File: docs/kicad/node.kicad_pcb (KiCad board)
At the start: 2 copper layers, 181.1 x 116.5 mm, 8 parts, among them J10 Conn_01x04_Pin, J11 Conn_01x04_Pin, J9 Conn_01x08, U1 ESP32-DevKitC, U2 ESP32-DevKitC, U3 ESP32-DevKitC, U4 ESP32-DevKitC, U5 ESP32-DevKitC

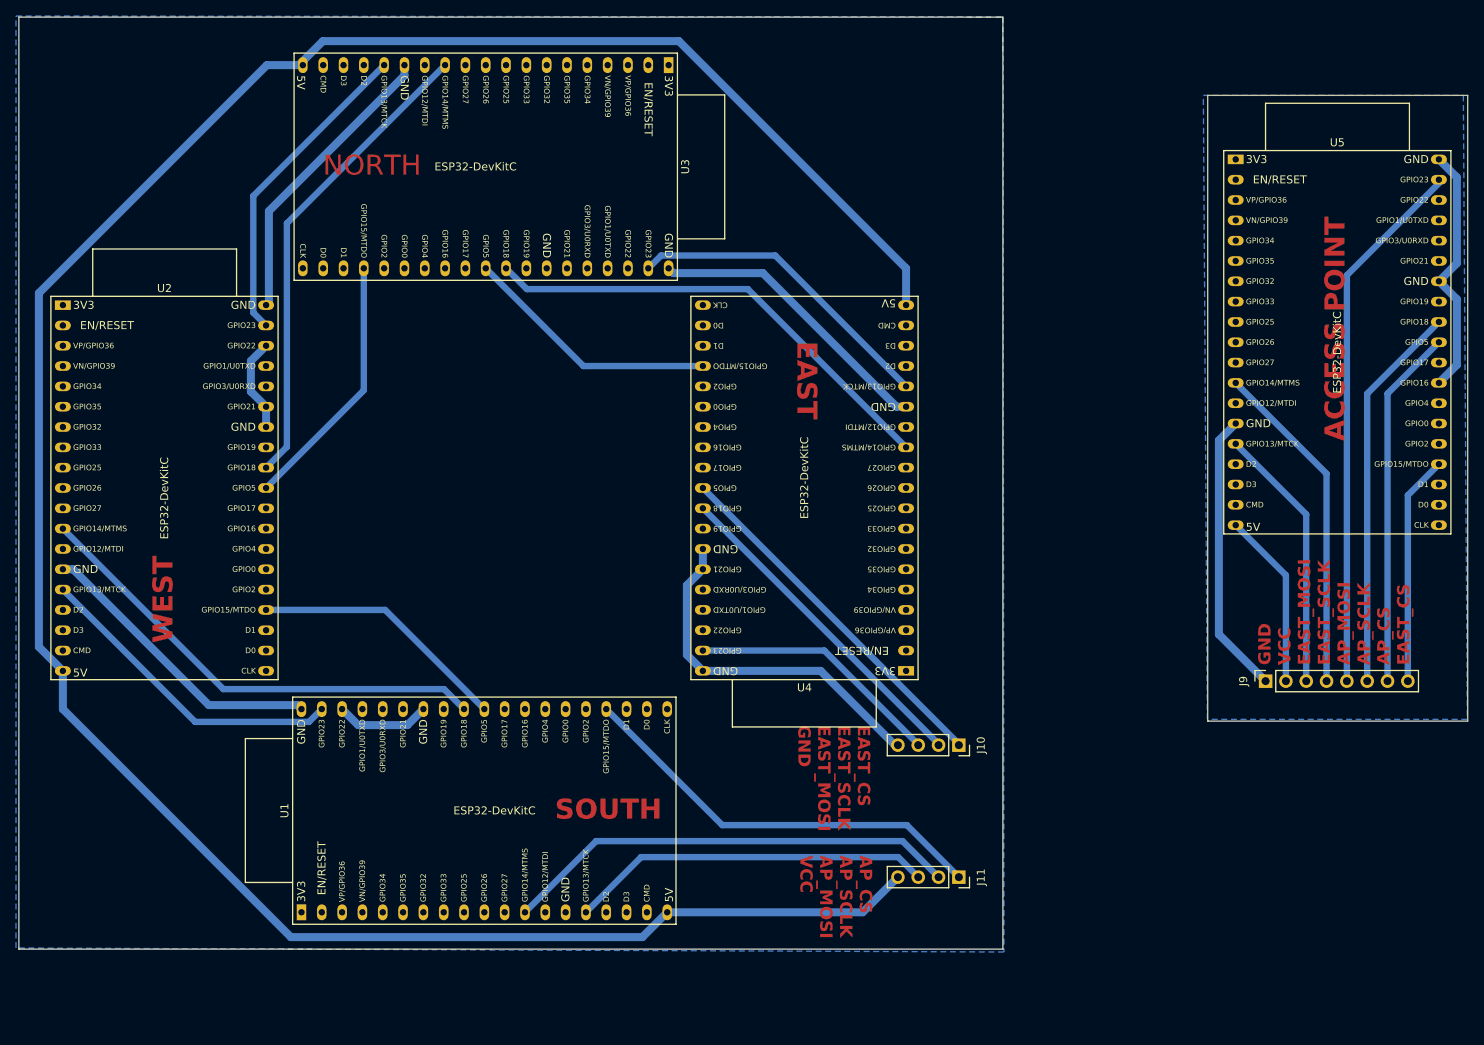
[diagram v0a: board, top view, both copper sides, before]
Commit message: resolved all errors
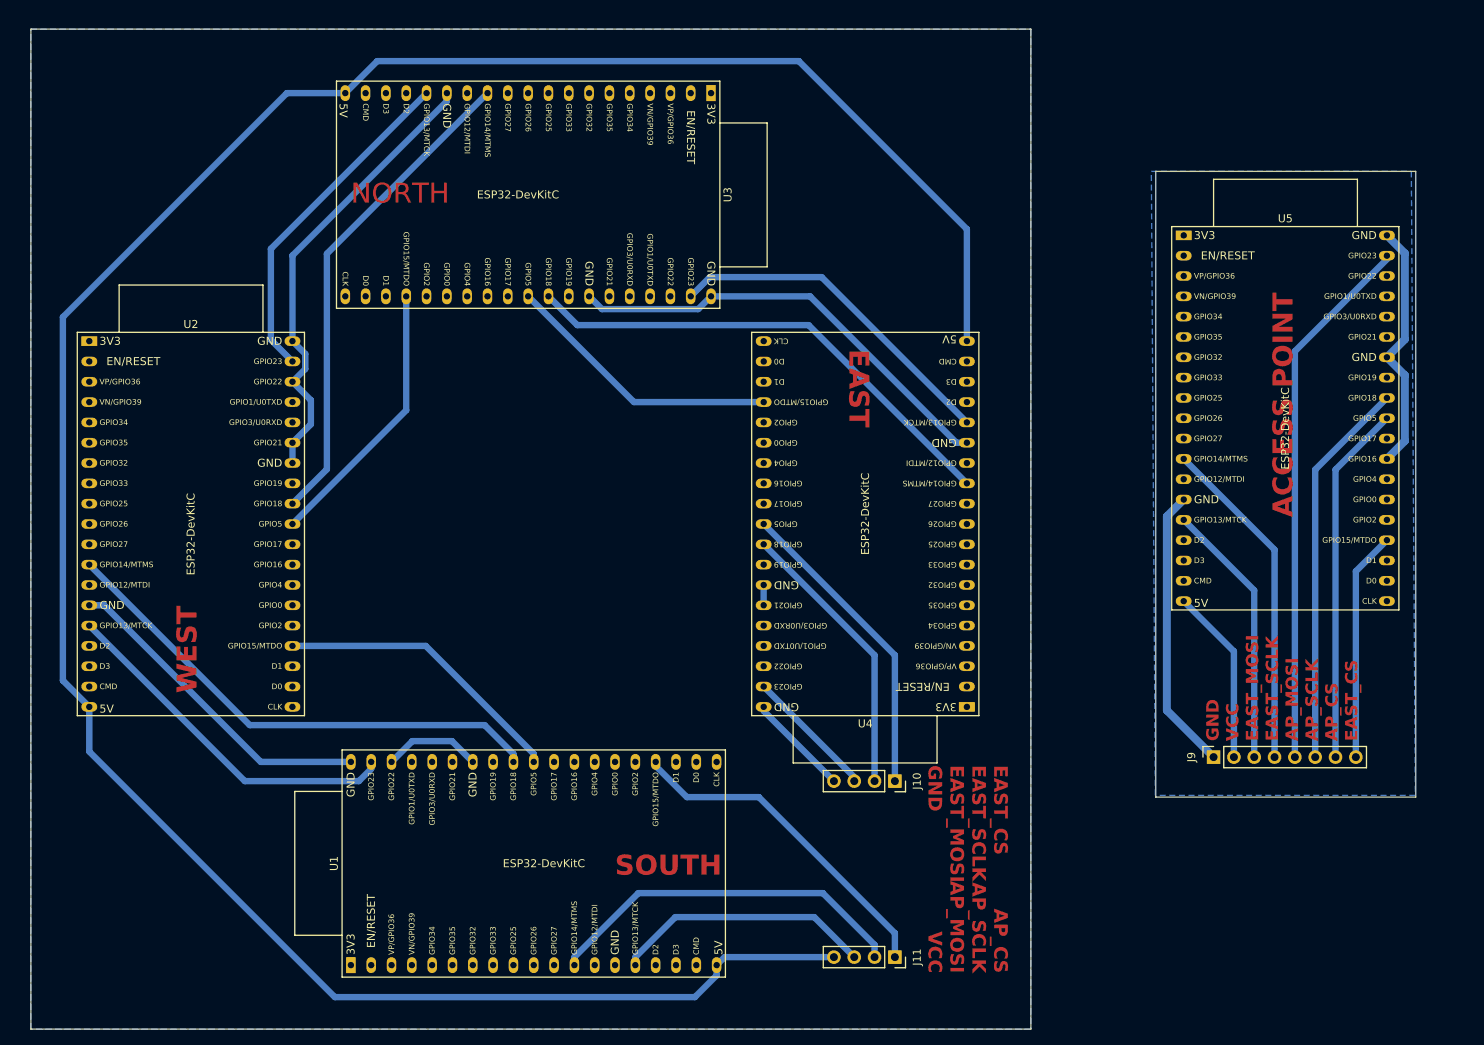
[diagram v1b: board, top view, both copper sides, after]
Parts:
- moved J11 12.8 mm to (122.0, 130.0)
- moved J9 11.5 mm to (161.8, 105.0)
- moved U5 11.5 mm to (158.1, 39.8)
- moved J10 9.18 mm to (122.0, 108.0)
- moved U1 9.04 mm to (54.0, 131.0)
- moved U4 8.83 mm to (131.0, 98.7)
- moved U3 6.35 mm to (99.0, 22.0)
- moved U2 5.58 mm to (21.3, 53.0)
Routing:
- net /main/B4_MOSI: track 31.9 -> 16.5 mm
- net /main/B5_MOSI: track 45.4 -> 32.5 mm
- net /main/B5_SCLK: track 57.2 -> 46.0 mm
- net /main/B5_CS: track 52.8 -> 42.1 mm
- net /main/B4_SCLK: track 41.8 -> 35.5 mm
- net /main/B4_CS: track 45.4 -> 39.1 mm
- net /main/B1_MOSI: track 39.9 -> 44.8 mm
- net /main/B1_SCLK: track 59.5 -> 63.8 mm
- net /main/B1_CS: track 32.4 -> 36.8 mm
- net /main/B3_MOSI: track 39.7 -> 43.0 mm
- net /main/B2_MOSI: track 40.0 -> 42.7 mm
- net /main/B3_CS: track 32.2 -> 34.9 mm
- net /main/B3_SCLK: track 59.3 -> 62.0 mm
- net GND: track 179.7 -> 182.2 mm
- net /main/VCC: track 310.8 -> 313.2 mm
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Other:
- board size 181.1 x 116.5 mm -> 173.1 x 125 mm
